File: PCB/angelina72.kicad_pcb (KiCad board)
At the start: 2 copper layers, 176.4 x 111.6 mm, 87 parts, among them J1 MJ-4PP-9, J2 LED, SW1 KEY_SWITCH, SW10 KEY_SWITCH, SW11 KEY_SWITCH, SW12 KEY_SWITCH, SW13 KEY_SWITCH, SW14 KEY_SWITCH, SW15 KEY_SWITCH, SW16 KEY_SWITCH, SW17 KEY_SWITCH, SW18 KEY_SWITCH, SW19 KEY_SWITCH, SW2 KEY_SWITCH, SW20 KEY_SWITCH, SW21 KEY_SWITCH, SW22 KEY_SWITCH, SW23 KEY_SWITCH, SW24 KEY_SWITCH, SW25 KEY_SWITCH, SW26 KEY_SWITCH, SW27 KEY_SWITCH, SW28 KEY_SWITCH, SW29 KEY_SWITCH, SW3 KEY_SWITCH, SW30 KEY_SWITCH, SW31 KEY_SWITCH, SW32 KEY_SWITCH, SW33 KEY_SWITCH, SW34 KEY_SWITCH, SW35 KEY_SWITCH, SW36 KEY_SWITCH, SW4 KEY_SWITCH, SW5 KEY_SWITCH, SW6 KEY_SWITCH, SW7 KEY_SWITCH, SW8 KEY_SWITCH, SW9 KEY_SWITCH, U1 ProMicro

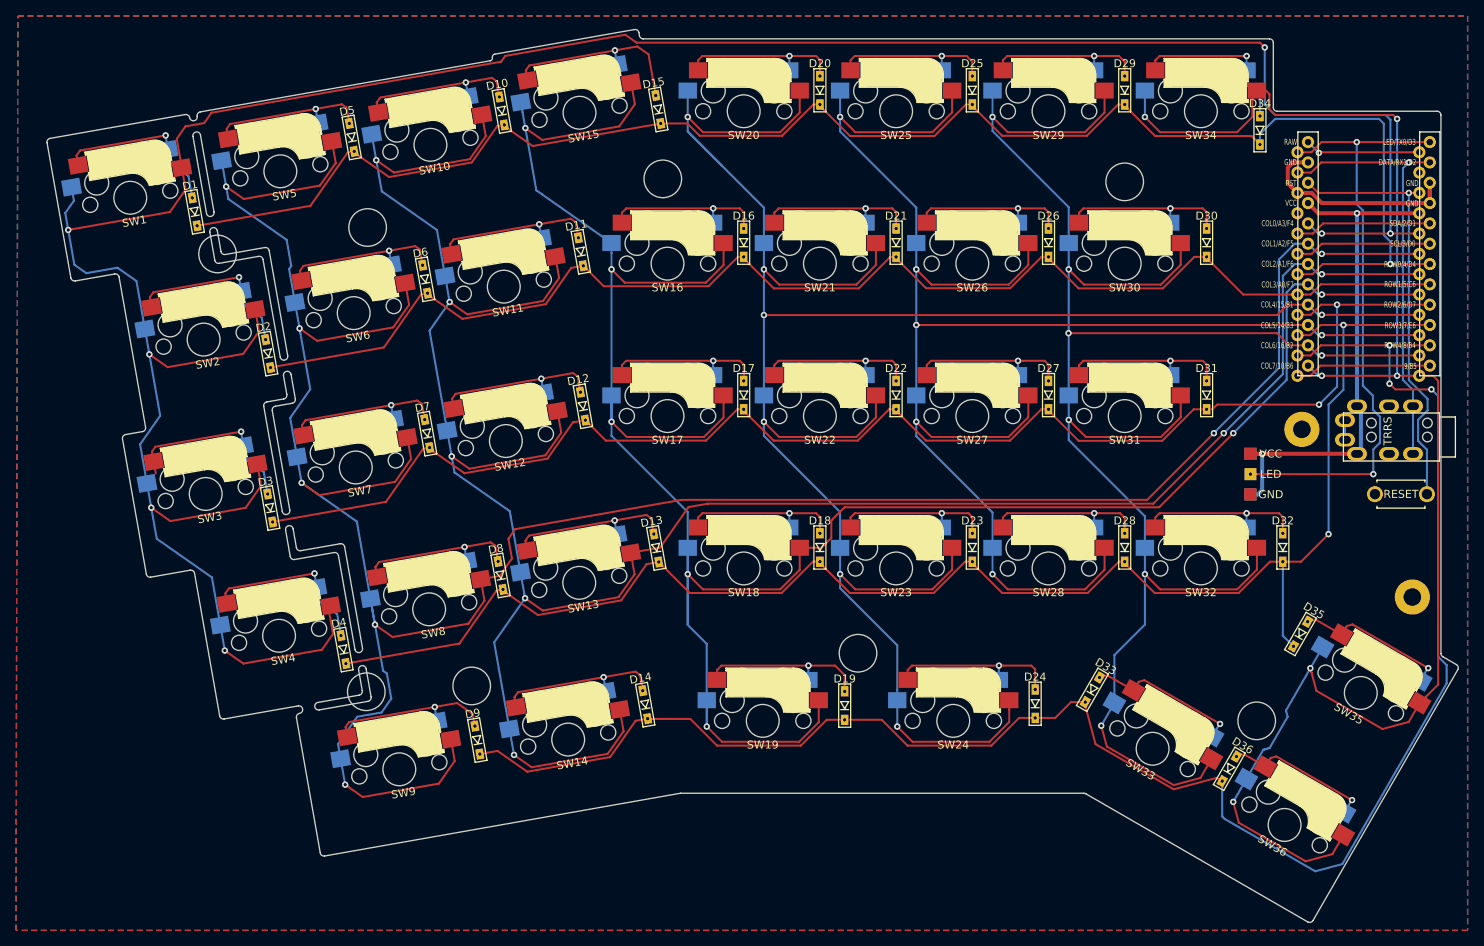
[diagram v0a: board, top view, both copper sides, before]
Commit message: Update PCBs
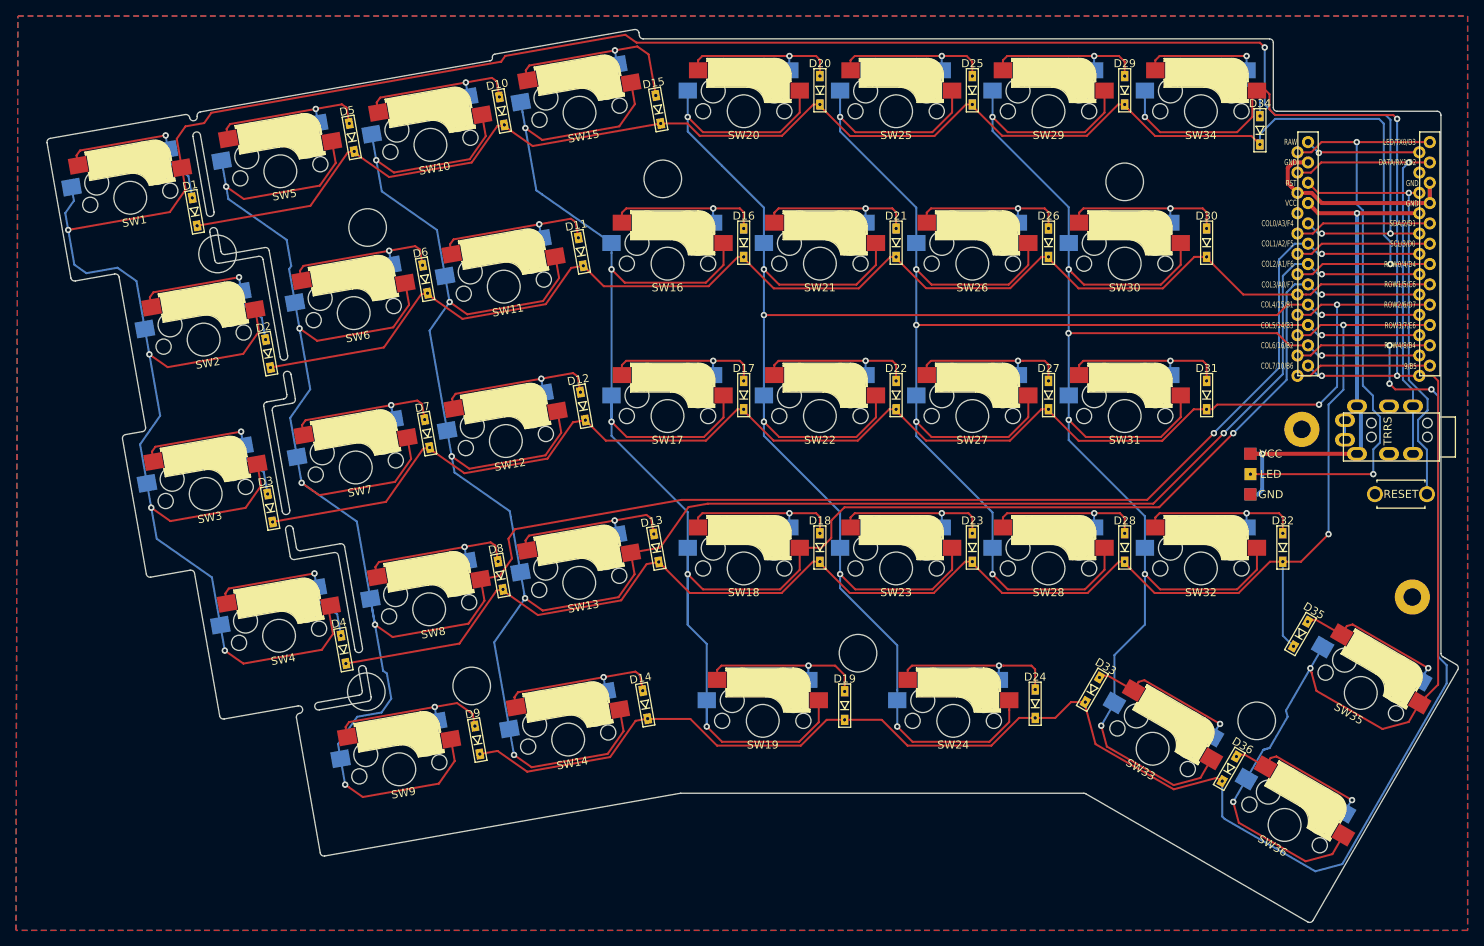
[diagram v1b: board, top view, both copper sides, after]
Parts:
- added REF**: Layout_Outline_PromicroBase, angelina72:Layout_Outline_PromicroBase, F.Cu at (113.2, 113.0)
- added REF**: Layout_Outline, angelina72:Layout_Outline, F.Cu at (113.2, 113.0)
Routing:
- net col4: track 275.3 -> 269.2 mm
- net Net-(D3-Pad2): track 23.5 -> 22.0 mm
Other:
- outline, holes or cut-outs redrawn
